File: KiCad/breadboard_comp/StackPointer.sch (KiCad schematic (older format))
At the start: 15 parts, among them U22 74LS08, U72 74LS245, U73 74LS169, U74 74LS08, U75 74LS245, U76 74LS157

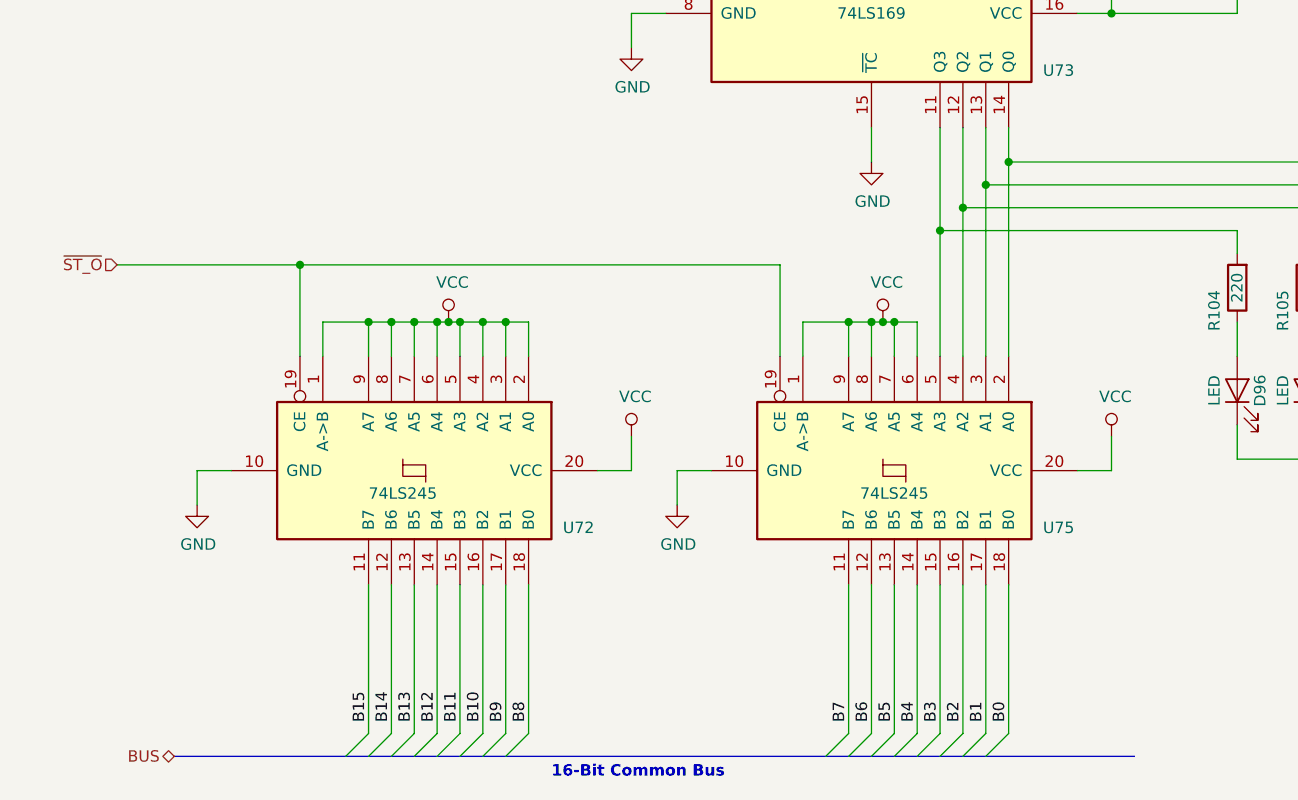
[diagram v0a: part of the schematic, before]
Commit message: Computer built
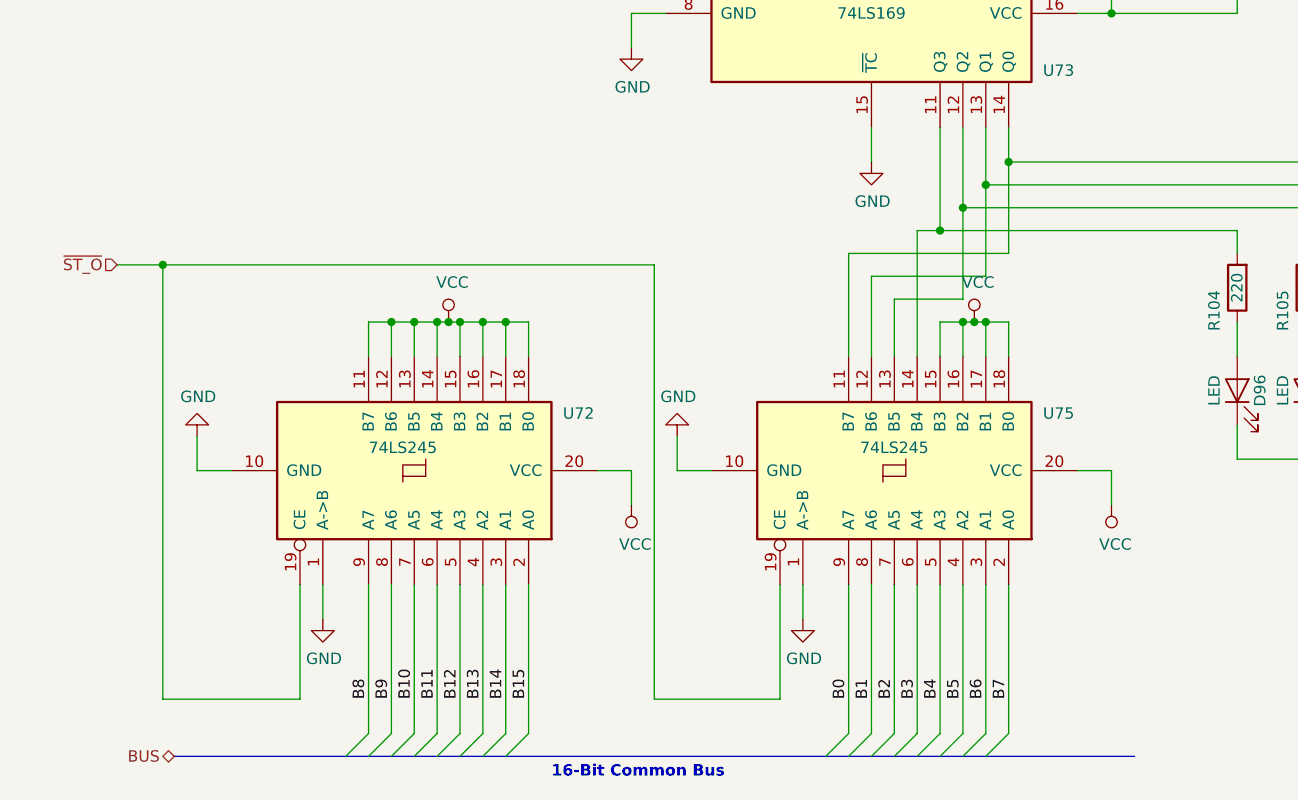
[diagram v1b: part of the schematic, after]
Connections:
- net B0: now also U75.9 (A7); no longer U75.18 (B0)
- net B1: now also U75.8 (A6); no longer U75.17 (B1)
- net B10: now also U72.7 (A5); no longer U72.16 (B2)
- net B11: now also U72.6 (A4); no longer U72.15 (B3)
- net B12: now also U72.5 (A3); no longer U72.14 (B4)
- net B13: now also U72.4 (A2); no longer U72.13 (B5)
- net B14: now also U72.3 (A1); no longer U72.12 (B6)
- net B15: now also U72.2 (A0); no longer U72.11 (B7)
- net B2: now also U75.7 (A5); no longer U75.16 (B2)
- net B3: now also U75.6 (A4); no longer U75.15 (B3)
- net B4: now also U75.5 (A3); no longer U75.14 (B4)
- net B5: now also U75.4 (A2); no longer U75.13 (B5)
- net B6: now also U75.3 (A1); no longer U75.12 (B6)
- net B7: now also U75.2 (A0); no longer U75.11 (B7)
- net B8: now also U72.9 (A7); no longer U72.18 (B0)
- net B9: now also U72.8 (A6); no longer U72.17 (B1)
- net GND: now also U72.1 (A->B), U75.1 (A->B)
- net VCC: now also U72.11 (B7), U72.12 (B6), U72.13 (B5), U72.14 (B4), U72.15 (B3), U72.16 (B2), U72.17 (B1), U72.18 (B0), U75.15 (B3), U75.16 (B2), U75.17 (B1), U75.18 (B0); no longer U72.1 (A->B), U72.2 (A0), U72.3 (A1), U72.4 (A2), U72.5 (A3), U72.6 (A4), U72.7 (A5), U72.8 (A6), U72.9 (A7), U75.1 (A->B), U75.6 (A4), U75.7 (A5), U75.8 (A6), U75.9 (A7)
- net at R104.2, U73.11 (Q3): now also U75.14 (B4); no longer U75.5 (A3)
- net at R105.2, U73.12 (Q2): now also U75.13 (B5); no longer U75.4 (A2)
- net at R106.2, U73.13 (Q1): now also U75.12 (B6); no longer U75.3 (A1)
- net at R107.2, U73.14 (Q0): now also U75.11 (B7); no longer U75.2 (A0)
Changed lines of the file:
@@
 $Descr A4 11693 8268
 encoding utf-8
-Sheet 15 18
+Sheet 14 18
 Title ""
 Date ""
@@
 F 3 "http://www.ti.com/lit/gpn/sn74LS245" H 4500 5650 50  0001 C CNN
 	1    4500 5650
-	0    1    1    0
+	0    1    -1   0
 $EndComp
 $Comp
@@
 F 3 "http://www.ti.com/lit/gpn/sn74LS245" H 2400 5650 50  0001 C CNN
 	1    2400 5650
-	0    1    1    0
+	0    1    -1   0
 $EndComp
 $Comp
 L power:VCC #PWR0184
 U 1 1 5E75594C
-P 4450 5000
-F 0 "#PWR0184" H 4450 4850 50  0001 C CNN
-F 1 "VCC" H 4467 5173 50  0000 C CNN
-F 2 "" H 4450 5000 50  0001 C CNN
-F 3 "" H 4450 5000 50  0001 C CNN
-	1    4450 5000
-	1    0    0    -1
-$EndComp
-Wire Wire Line
-	4450 5000 4400 5000
-Wire Wire Line
-	4300 5000 4300 5150
-Wire Wire Line
-	4400 5150 4400 5000
-Connection ~ 4400 5000
-Wire Wire Line
-	4400 5000 4300 5000
-Wire Wire Line
-	4450 5000 4500 5000
-Wire Wire Line
-	4600 5000 4600 5150
-Connection ~ 4450 5000
-Wire Wire Line
-	4500 5150 4500 5000
-Connection ~ 4500 5000
-Wire Wire Line
-	4500 5000 4600 5000
+P 4850 5000
+F 0 "#PWR0184" H 4850 4850 50  0001 C CNN
+F 1 "VCC" H 4867 5173 50  0000 C CNN
+F 2 "" H 4850 5000 50  0001 C CNN
+F 3 "" H 4850 5000 50  0001 C CNN
+	1    4850 5000
+	1    0    0    -1
+$EndComp
+Wire Wire Line
+	4850 5000 4800 5000
+Wire Wire Line
+	4700 5000 4700 5150
+Wire Wire Line
+	4800 5150 4800 5000
+Connection ~ 4800 5000
+Wire Wire Line
+	4800 5000 4700 5000
+Wire Wire Line
+	4850 5000 4900 5000
+Wire Wire Line
+	5000 5000 5000 5150
+Connection ~ 4850 5000
+Wire Wire Line
+	4900 5150 4900 5000
+Connection ~ 4900 5000
+Wire Wire Line
+	4900 5000 5000 5000
 $Comp
 L power:VCC #PWR0179
@@
 L power:VCC #PWR0181
 U 1 1 5E767A05
-P 3350 5500
-F 0 "#PWR0181" H 3350 5350 50  0001 C CNN
-F 1 "VCC" H 3367 5673 50  0000 C CNN
-F 2 "" H 3350 5500 50  0001 C CNN
-F 3 "" H 3350 5500 50  0001 C CNN
-	1    3350 5500
-	1    0    0    -1
+P 3350 5800
+F 0 "#PWR0181" H 3350 5650 50  0001 C CNN
+F 1 "VCC" H 3367 5973 50  0000 C CNN
+F 2 "" H 3350 5800 50  0001 C CNN
+F 3 "" H 3350 5800 50  0001 C CNN
+	1    3350 5800
+	1    0    0    1
 $EndComp
 $Comp
 L power:GND #PWR0178
 U 1 1 5E767B94
-P 1450 5800
-F 0 "#PWR0178" H 1450 5550 50  0001 C CNN
-F 1 "GND" H 1455 5627 50  0000 C CNN
-F 2 "" H 1450 5800 50  0001 C CNN
-F 3 "" H 1450 5800 50  0001 C CNN
-	1    1450 5800
-	1    0    0    -1
+P 1450 5500
+F 0 "#PWR0178" H 1450 5250 50  0001 C CNN
+F 1 "GND" H 1455 5327 50  0000 C CNN
+F 2 "" H 1450 5500 50  0001 C CNN
+F 3 "" H 1450 5500 50  0001 C CNN
+	1    1450 5500
+	1    0    0    1
 $EndComp
 $Comp
 L power:GND #PWR0182
 U 1 1 5E767D00
-P 3550 5800
-F 0 "#PWR0182" H 3550 5550 50  0001 C CNN
-F 1 "GND" H 3555 5627 50  0000 C CNN
-F 2 "" H 3550 5800 50  0001 C CNN
-F 3 "" H 3550 5800 50  0001 C CNN
-	1    3550 5800
-	1    0    0    -1
+P 3550 5500
+F 0 "#PWR0182" H 3550 5250 50  0001 C CNN
+F 1 "GND" H 3555 5327 50  0000 C CNN
+F 2 "" H 3550 5500 50  0001 C CNN
+F 3 "" H 3550 5500 50  0001 C CNN
+	1    3550 5500
+	1    0    0    1
 $EndComp
 $Comp
 L power:VCC #PWR0186
 U 1 1 5E767EA3
-P 5450 5500
-F 0 "#PWR0186" H 5450 5350 50  0001 C CNN
-F 1 "VCC" H 5467 5673 50  0000 C CNN
-F 2 "" H 5450 5500 50  0001 C CNN
-F 3 "" H 5450 5500 50  0001 C CNN
-	1    5450 5500
-	1    0    0    -1
-$EndComp
-Wire Wire Line
-	5450 5500 5450 5650
+P 5450 5800
+F 0 "#PWR0186" H 5450 5650 50  0001 C CNN
+F 1 "VCC" H 5467 5973 50  0000 C CNN
+F 2 "" H 5450 5800 50  0001 C CNN
+F 3 "" H 5450 5800 50  0001 C CNN
+	1    5450 5800
+	1    0    0    1
+$EndComp
+Wire Wire Line
+	5450 5800 5450 5650
 Wire Wire Line
 	5450 5650 5300 5650
@@
 	3700 5650 3550 5650
 Wire Wire Line
-	3550 5650 3550 5800
+	3550 5650 3550 5500
 Wire Wire Line
 	3200 5650 3350 5650
 Wire Wire Line
-	3350 5650 3350 5500
+	3350 5650 3350 5800
 Wire Wire Line
 	1600 5650 1450 5650
 Wire Wire Line
-	1450 5650 1450 5800
-Wire Wire Line
-	5000 5150 5000 4300
+	1450 5650 1450 5500
 Wire Wire Line
 	4900 4150 4900 4400
 Wire Wire Line
-	4800 5150 4800 4500
-Wire Wire Line
-	1900 5150 1900 4750
-Wire Wire Line
-	1900 4750 4000 4750
-Wire Wire Line
-	4000 4750 4000 5150
-Wire Wire Line
-	1100 4750 1900 4750
-Connection ~ 1900 4750
-Wire Wire Line
-	2000 5150 2000 5000
-Wire Wire Line
-	2000 5000 2200 5000
-Connection ~ 2200 5000
-Wire Wire Line
 	2200 5000 2300 5000
-Wire Wire Line
-	4300 5000 4100 5000
-Wire Wire Line
-	4100 5000 4100 5150
-Connection ~ 4300 5000
 Wire Wire Line
 	4500 2150 4500 3150
@@
 Wire Wire Line
 	6000 4600 4700 4600
-Connection ~ 4700 4600
-Wire Wire Line
-	4700 4600 4700 5150
 Wire Wire Line
 	4800 4500 6300 4500
 Wire Wire Line
 	6300 4500 6300 4700
-Connection ~ 4800 4500
 Wire Wire Line
 	4800 4500 4800 4150
@@
 Wire Wire Line
 	6600 4400 4900 4400
-Connection ~ 4900 4400
-Wire Wire Line
-	4900 4400 4900 5150
 Wire Wire Line
 	5000 4300 6900 4300
 Wire Wire Line
 	6900 4300 6900 4700
-Connection ~ 5000 4300
 Wire Wire Line
 	5000 4300 5000 4150
@@
 	1    0    0    -1
 $EndComp
-Text Label 5000 6750 1    50   ~ 0
+Text Label 4300 6650 1    50   ~ 0
 B0
-Text Label 4900 6750 1    50   ~ 0
+Text Label 4400 6650 1    50   ~ 0
 B1
-Text Label 4800 6750 1    50   ~ 0
+Text Label 4500 6650 1    50   ~ 0
 B2
-Text Label 4700 6750 1    50   ~ 0
+Text Label 4600 6650 1    50   ~ 0
 B3
-Text Label 4600 6750 1    50   ~ 0
+Text Label 4700 6650 1    50   ~ 0
 B4
-Text Label 4500 6750 1    50   ~ 0
+Text Label 4800 6650 1    50   ~ 0
 B5
-Text Label 4400 6750 1    50   ~ 0
+Text Label 4900 6650 1    50   ~ 0
 B6
-Text Label 4300 6750 1    50   ~ 0
+Text Label 5000 6650 1    50   ~ 0
 B7
-Text Label 2900 6750 1    50   ~ 0
+Text Label 2200 6650 1    50   ~ 0
 B8
-Text Label 2800 6750 1    50   ~ 0
+Text Label 2300 6650 1    50   ~ 0
 B9
-Text Label 2700 6750 1    50   ~ 0
+Text Label 2400 6650 1    50   ~ 0
 B10
-Text Label 2600 6750 1    50   ~ 0
+Text Label 2500 6650 1    50   ~ 0
 B11
-Text Label 2500 6750 1    50   ~ 0
+Text Label 2600 6650 1    50   ~ 0
 B12
-Text Label 2400 6750 1    50   ~ 0
+Text Label 2700 6650 1    50   ~ 0
 B13
-Text Label 2300 6750 1    50   ~ 0
+Text Label 2800 6650 1    50   ~ 0
 B14
-Text Label 2200 6750 1    50   ~ 0
+Text Label 2900 6650 1    50   ~ 0
 B15
 Text HLabel 1350 6900 0    50   BiDi ~ 0
@@
 Wire Bus Line
 	9050 1800 8850 1800
+Wire Wire Line
+	5000 4300 5000 4700
+Wire Wire Line
+	5000 4700 4300 4700
+Wire Wire Line
+	4300 4700 4300 5150
+Connection ~ 5000 4300
+Wire Wire Line
+	4400 5150 4400 4800
+Wire Wire Line
+	4400 4800 4900 4800
+Wire Wire Line
+	4900 4800 4900 4400
+Connection ~ 4900 4400
+Wire Wire Line
+	4800 4500 4800 4900
+Wire Wire Line
+	4800 4900 4500 4900
+Wire Wire Line
+	4500 4900 4500 5150
+Connection ~ 4800 4500
+Wire Wire Line
+	4600 5150 4600 4600
+Wire Wire Line
+	4600 4600 4700 4600
+Connection ~ 4700 4600
+Wire Wire Line
+	1100 4750 1300 4750
+Wire Wire Line
+	3450 4750 3450 6650
+Wire Wire Line
+	3450 6650 4000 6650
+Wire Wire Line
+	4000 6150 4000 6650
+Wire Wire Line
+	1900 6150 1900 6650
+Wire Wire Line
+	1900 6650 1300 6650
+Wire Wire Line
+	1300 6650 1300 4750
+Connection ~ 1300 4750
+Wire Wire Line
+	1300 4750 3450 4750
+$Comp
+L power:GND #PWR0148
+U 1 1 5EB75D42
+P 2000 6300
+F 0 "#PWR0148" H 2000 6050 50  0001 C CNN
+F 1 "GND" H 2005 6127 50  0000 C CNN
+F 2 "" H 2000 6300 50  0001 C CNN
+F 3 "" H 2000 6300 50  0001 C CNN
+	1    2000 6300
+	1    0    0    -1
+$EndComp
+Wire Wire Line
+	2000 6300 2000 6150
+$Comp
+L power:GND #PWR0259
+U 1 1 5EB7CBD9
+P 4100 6300
+F 0 "#PWR0259" H 4100 6050 50  0001 C CNN
+F 1 "GND" H 4105 6127 50  0000 C CNN
+F 2 "" H 4100 6300 50  0001 C CNN
+F 3 "" H 4100 6300 50  0001 C CNN
+	1    4100 6300
+	1    0    0    -1
+$EndComp
+Wire Wire Line
+	4100 6300 4100 6150
 Wire Bus Line
 	8850 1800 8850 3100

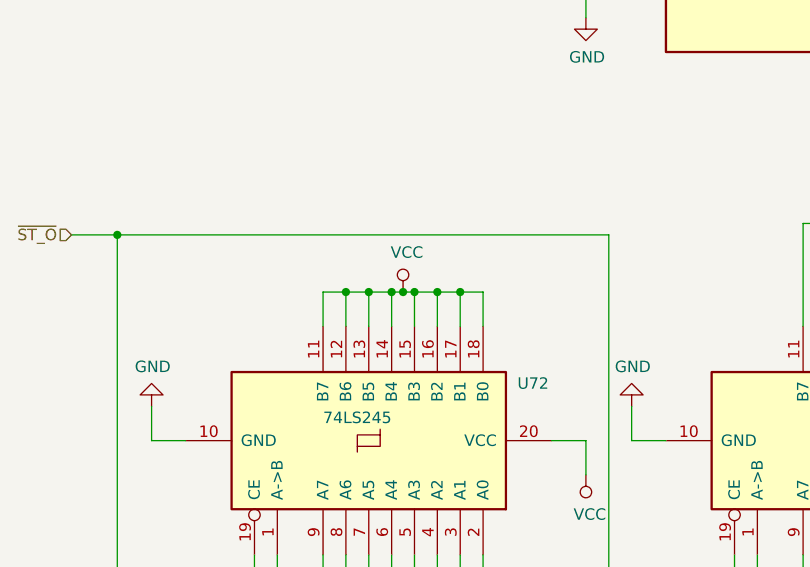
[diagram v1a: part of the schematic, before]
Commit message: Report Progress
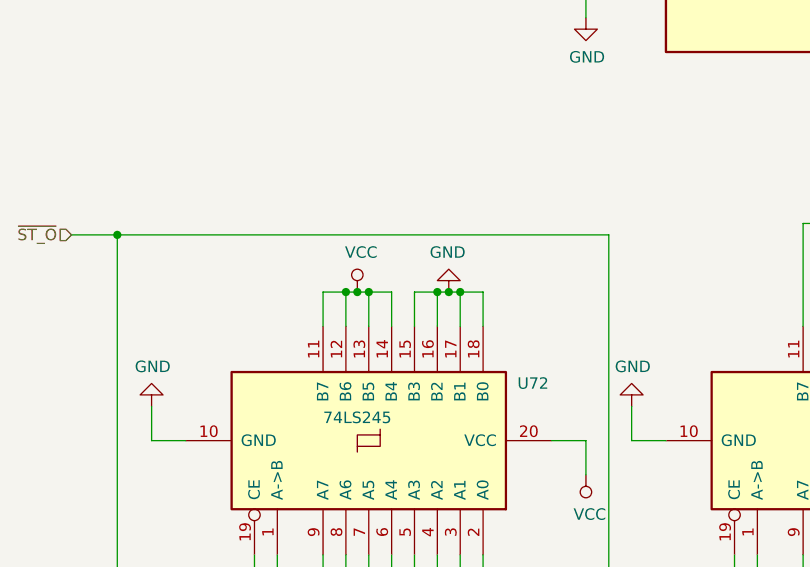
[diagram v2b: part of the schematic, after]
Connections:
- net GND: now also U72.15 (B3), U72.16 (B2), U72.17 (B1), U72.18 (B0)
- net VCC: no longer U72.15 (B3), U72.16 (B2), U72.17 (B1), U72.18 (B0)
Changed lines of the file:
@@
 L power:VCC #PWR0179
 U 1 1 5E7563C3
-P 2550 5000
-F 0 "#PWR0179" H 2550 4850 50  0001 C CNN
-F 1 "VCC" H 2567 5173 50  0000 C CNN
-F 2 "" H 2550 5000 50  0001 C CNN
-F 3 "" H 2550 5000 50  0001 C CNN
-	1    2550 5000
+P 2350 5000
+F 0 "#PWR0179" H 2350 4850 50  0001 C CNN
+F 1 "VCC" H 2367 5173 50  0000 C CNN
+F 2 "" H 2350 5000 50  0001 C CNN
+F 3 "" H 2350 5000 50  0001 C CNN
+	1    2350 5000
 	1    0    0    -1
 $EndComp
 Wire Wire Line
-	2550 5000 2600 5000
-Wire Wire Line
-	2900 5000 2900 5150
-Wire Wire Line
 	2200 5150 2200 5000
-Connection ~ 2550 5000
 Wire Wire Line
 	2300 5150 2300 5000
 Connection ~ 2300 5000
 Wire Wire Line
-	2300 5000 2400 5000
+	2300 5000 2350 5000
 Wire Wire Line
 	2400 5000 2400 5150
@@
 Wire Wire Line
 	2500 5150 2500 5000
-Connection ~ 2500 5000
-Wire Wire Line
-	2500 5000 2550 5000
-Wire Wire Line
-	2600 5000 2600 5150
-Connection ~ 2600 5000
-Wire Wire Line
-	2600 5000 2700 5000
-Wire Wire Line
-	2700 5150 2700 5000
-Connection ~ 2700 5000
-Wire Wire Line
-	2700 5000 2800 5000
-Wire Wire Line
-	2800 5000 2800 5150
-Connection ~ 2800 5000
-Wire Wire Line
-	2800 5000 2900 5000
 Text Notes 3000 7000 0    50   ~ 10
 16-Bit Common Bus\n
@@
 Wire Wire Line
 	4100 6300 4100 6150
+Connection ~ 2350 5000
+Wire Wire Line
+	2350 5000 2400 5000
+Wire Wire Line
+	2600 5150 2600 5000
+Wire Wire Line
+	2600 5000 2700 5000
+Wire Wire Line
+	2900 5000 2900 5150
+Wire Wire Line
+	2800 5150 2800 5000
+Connection ~ 2800 5000
+Wire Wire Line
+	2800 5000 2900 5000
+Wire Wire Line
+	2700 5000 2700 5150
 Wire Bus Line
 	8850 1800 8850 3100
 Wire Bus Line
 	1350 6900 5550 6900
+Connection ~ 2700 5000
+Wire Wire Line
+	2700 5000 2750 5000
+$Comp
+L power:GND #PWR?
+U 1 1 5FFAD838
+P 2750 5000
+F 0 "#PWR?" H 2750 4750 50  0001 C CNN
+F 1 "GND" H 2755 4827 50  0000 C CNN
+F 2 "" H 2750 5000 50  0001 C CNN
+F 3 "" H 2750 5000 50  0001 C CNN
+	1    2750 5000
+	-1   0    0    1
+$EndComp
+Connection ~ 2750 5000
+Wire Wire Line
+	2750 5000 2800 5000
 $EndSCHEMATC
